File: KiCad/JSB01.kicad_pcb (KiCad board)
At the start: 2 copper layers, 88 x 33 mm, 35 parts, among them J1 MB10XX Sonar, J2 VL53LXX TOF(0x29), M1 LD14, Q2 AO3400A, SW1 Tactile, SW2 Tactile, SW3 Slide, U1 TPS61291DRVR, U2 QMC5883L(0x0D), U3 BH1750FVI(0x23)

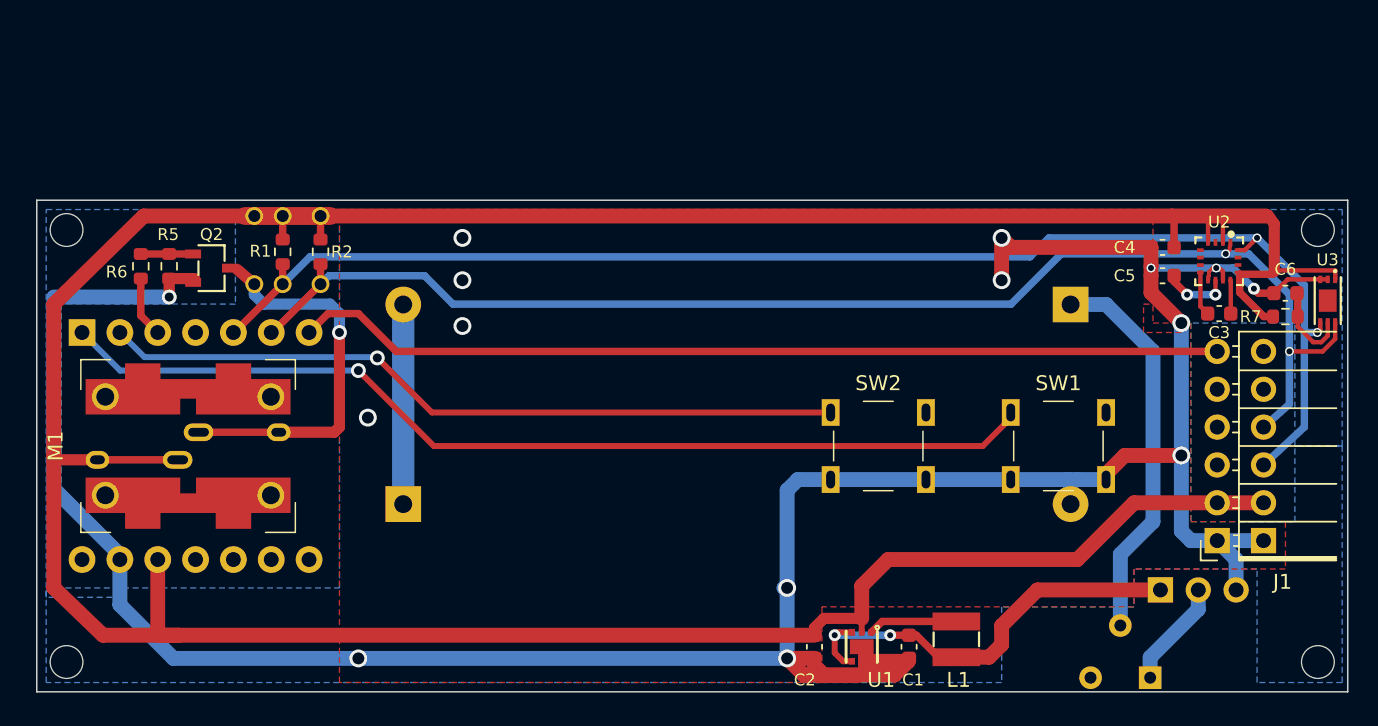
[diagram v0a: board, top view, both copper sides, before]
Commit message: BTO ver. (QMC5883P)
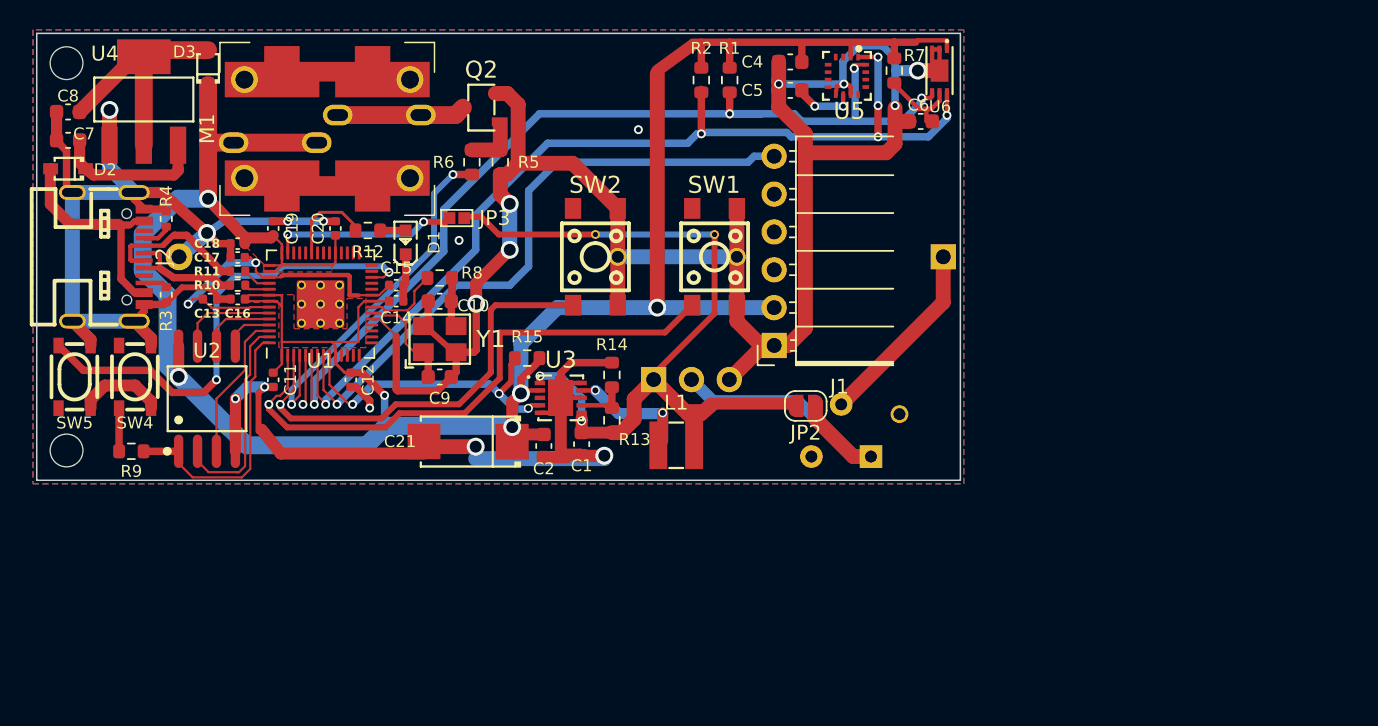
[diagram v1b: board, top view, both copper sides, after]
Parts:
- removed C3: 0.22uF, Capacitor_SMD:C_0603_1608Metric
- removed MCU1: XIAO RP2040, JSB01_Lib:MOUDLE14P-2.54-21X17.8MM
- removed the Pad at (41.9, 39.9)
- removed the Pad at (44.5, 35.4)
- removed the Pad at (40.0, 39.9)
- removed the Pad at (44.5, 39.9)
- removed the Pad at (41.9, 35.4)
- removed the Pad at (40.0, 35.4)
- removed the REF** at (27.4, 65.3)
- removed the REF** at (111.4, 65.3)
- removed the REF** at (27.4, 36.3)
- removed the REF** at (111.4, 36.3)
- added ?: , , F.Cu at (83.3, 48.8)
- added C10: 33p, Capacitor_SMD:C_0603_1608Metric, F.Cu at (52.5, 41.1)
- added C11: 100n, Capacitor_SMD:C_0402_1005Metric, F.Cu at (41.3, 46.4)
- added C12: 100n, Capacitor_SMD:C_0402_1005Metric, F.Cu at (46.5, 46.4)
- added C13: 100n, Capacitor_SMD:C_0402_1005Metric, F.Cu at (37.0, 40.9)
- added C14: 100n, Capacitor_SMD:C_0402_1005Metric, F.Cu at (49.5, 41.1)
- added C15: 100n, Capacitor_SMD:C_0402_1005Metric, F.Cu at (49.5, 40.0)
- added C16: 100n, Capacitor_SMD:C_0402_1005Metric, F.Cu at (38.9, 40.9)
- added C17: 100n, Capacitor_SMD:C_0402_1005Metric, F.Cu at (38.9, 38.1)
- added C18: 100n, Capacitor_SMD:C_0402_1005Metric, F.Cu at (38.9, 37.2)
- added C19: 100n, Capacitor_SMD:C_0402_1005Metric, F.Cu at (41.3, 36.2)
- added C20: 100n, Capacitor_SMD:C_0402_1005Metric, F.Cu at (45.5, 36.2)
- added C21: 100u, JSB01_Lib:CAP-SMD_L6.0-W3.2, F.Cu at (54.4, 50.5)
- added C7: 10u, Capacitor_SMD:C_0603_1608Metric, F.Cu at (27.5, 30.3)
- added C8: 10u, Capacitor_SMD:C_0603_1608Metric, F.Cu at (27.5, 28.4)
- added C9: 33p, Capacitor_SMD:C_0603_1608Metric, F.Cu at (52.5, 46.2)
- added D1: LED, JSB01_Lib:LED0603-RD_GREEN, F.Cu at (50.2, 37.1)
- added D2: NSR0320MW2T1G, JSB01_Lib:SOD-323_L1.8-W1.3-LS2.5-RD, F.Cu at (27.5, 32.2)
- added D3: 1N5819WS, JSB01_Lib:SOD-323_L1.8-W1.3-LS2.5-RD, F.Cu at (36.9, 25.4)
- added JP2: SolderJumper_2_Open, Jumper:SolderJumper-2_P1.3mm_Open_RoundedPad1.0x1.5mm, F.Cu at (77.0, 48.1)
- added JP3: SolderJumper_2_Open, JSB01_Lib:SolderJumper-2_Open_mini, F.Cu at (53.6, 35.5)
- added Pad: Pad1.2_0.8, JSB01_Lib:Pad1.2_0.8, F.Cu at (71.1, 38.1)
- added Pad: Pad0.6_0.35, JSB01_Lib:Pad0.6_0.35, F.Cu at (62.5, 36.6)
- added Pad: Pad0.6_0.35, JSB01_Lib:Pad0.6_0.35, F.Cu at (70.6, 36.6)
- added Pad: Pad1.2_0.8, JSB01_Lib:Pad1.2_0.8, F.Cu at (63.0, 38.1)
- added R10: 27.4, Resistor_SMD:R_0402_1005Metric, F.Cu at (38.9, 40.0)
- added R11: 27.4, Resistor_SMD:R_0402_1005Metric, F.Cu at (38.9, 39.1)
- added R12: 470, Resistor_SMD:R_0603_1608Metric, F.Cu at (47.6, 36.3)
- added R13: 470K, Resistor_SMD:R_0603_1608Metric, F.Cu at (64.0, 49.1)
- added R14: 390K, Resistor_SMD:R_0603_1608Metric, F.Cu at (64.0, 46.0)
- added R15: 1M, Resistor_SMD:R_0603_1608Metric, F.Cu at (58.3, 44.9)
- added R3: 5.1K, Resistor_SMD:R_0402_1005Metric, F.Cu at (34.1, 40.6)
- added R4: 5.1K, Resistor_SMD:R_0402_1005Metric, F.Cu at (34.1, 35.6)
- added R8: 1K, Resistor_SMD:R_0603_1608Metric, F.Cu at (52.5, 39.5)
- added R9: 1k, Resistor_SMD:R_0603_1608Metric, F.Cu at (31.8, 51.2)
- added REF**: MountingHole_2.2mm_M2, MountingHole:MountingHole_2.2mm_M2, F.Cu at (27.4, 25.1)
- added REF**: MountingHole_2.2mm_M2, MountingHole:MountingHole_2.2mm_M2, F.Cu at (27.4, 51.1)
- added SW4: SKRPABE010, JSB01_Lib:KEY-SMD_4P-L4.2-W3.2, F.Cu at (32.0, 46.2)
- added SW5: SKRPABE010, JSB01_Lib:KEY-SMD_4P-L4.2-W3.2, F.Cu at (27.9, 46.2)
- added U3: TPS61025DRCR, JSB01_Lib:VSON-10_L3.0-W3.0-P0.50-BL-EP, F.Cu at (60.6, 47.6)
- added U4: AMS1117-3.3, JSB01_Lib:SOT-223-3_L6.5-W3.4, F.Cu at (32.6, 27.6)
- added U5: QMC5883P(0x2C), JSB01_Lib:LGA-16_L3.0-W3.0-P0.50-BL_SQ, F.Cu at (79.8, 26.0)
- added Y1: TAXM12M4RLBDDT2T, JSB01_Lib:OSC-SMD_4P-L3.2-W2.5, F.Cu at (52.5, 43.6)
- BT1: value 2xAAA -> 1xAAA; footprint JSB01_Lib:BatteryHolder 2xAAA -> JSB01_Lib:BatteryHolder_SN4_1PC
- C1: value 10uF -> 10u
- C2: value 22uF -> 2.2u
- C4: value 0.1uF -> 0.1u
- C5: value 4.7uF -> 4.7u
- C6: value 1uF -> 1u
- J2: value VL53LXX TOF(0x29) -> USB_C_Receptacle_USB2.0; footprint Connector_PinSocket_2.54mm:PinSocket_1x06_P2.54mm_Vertical -> JSB01_Lib:USB-C-SMD_TYPE-C-16P-1; moved to F.Cu
- L1: value 3.3μH -> 6.8μH
- R1, R2: value 10KΩ -> 4.7K
- R5: value 100KΩ -> 100K
- R6: value 20KΩ -> 20K
- SW1, SW2: footprint JSB01_Lib:SW_tactile_DTS6 -> JSB01_Lib:SW-SMD_4P-L4.5-W4.5-P3.00-LS6.8
- U1: value TPS61291DRVR -> RP2040; footprint JSB01_Lib:WSON-6_L2.0-W2.0-P0.65-BL-EP -> JSB01_Lib:RP2040-QFN-56
- U2: value QMC5883L(0x0D) -> W25Q128JVSIQ; footprint JSB01_Lib:LGA-16_L3.0-W3.0-P0.50-BL_SQ -> JSB01_Lib:SOP-8-208mil
- moved J2 79.9 mm to (30.2, 38.1), turned to -90 degrees
- moved U2 68.6 mm to (36.8, 47.6), turned to 0 degrees
- moved U1 43.0 mm to (44.5, 41.3), turned to 90 degrees
- moved JP1 36.8 mm to (69.3, 46.3)
- moved J1 32.5 mm to (74.9, 37.7)
- moved R1 32.1 mm to (71.9, 26.2)
- moved R7 31.0 mm to (83.0, 25.6), turned to -90 degrees
- moved U6 30.3 mm to (86.0, 25.6)
- moved R2 28.0 mm to (70.0, 26.2)
- moved C4 27.9 mm to (76.0, 25.0)
- moved C5 27.9 mm to (76.0, 26.9)
- moved C6 27.1 mm to (84.7, 29.0)
- moved SW1 26.3 mm to (70.9, 38.1), turned to 90 degrees
- moved C1 25.8 mm to (62.0, 50.7)
- moved SW3 23.9 mm to (79.4, 49.8)
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- renumbered U3 to U6
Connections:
- C2 pad 1: +3.3V -> +3V3
- C4 pad 1: +3.3V -> +3V3
- C5 pad 1: Net-(U2-C1) -> Net-(U5-C1)
- J1 pad 2: +3.3V -> +3V3
- J1 pad 6: Net-(J1-PW) -> SONAR_PW
- L1 pad 2: Net-(U1-SW) -> Net-(U3-SW)
- M1 pad 1: +3.3V -> +3V3
- R1 pad 1: +3.3V -> +3V3
- R1 pad 2: Net-(J2-SDA) -> SDA
- R2 pad 1: +3.3V -> +3V3
- R2 pad 2: Net-(J2-SCL) -> SCL
- R6 pad 1: Net-(MCU1-D2) -> VIB
- R7 pad 1: +3.3V -> +3V3
- SW1 pad 1: Net-(MCU1-D0) -> SW1
- SW1 pad 2: GND -> SW1
- SW2 pad 1: Net-(MCU1-D1) -> SW2
- SW2 pad 2: GND -> SW2
- U1 pad 1: Net-(U1-SW) -> +3V3
- U1 pad 2: +3.3V -> SW1
- U1 pad 3: Net-(JP1-A) -> SW2
- U1 pad 4: Net-(JP1-A) -> VIB
- U1 pad 5: GND -> unconnected-(U1-GPIO3-Pad5)
- U1 pad 6: GND -> SDA
- U1 pad 7: GND -> SCL
- U2 pad 1: Net-(J2-SCL) -> QSPI_SS
- U2 pad 2: +3.3V -> QSPI_SD1
- U2 pad 3: unconnected-(U2-Pad3) -> QSPI_SD2
- U2 pad 4: +3.3V -> GND
- U2 pad 5: unconnected-(U2-Pad5) -> QSPI_SD0
- U2 pad 6: unconnected-(U2-Pad6) -> QSPI_SCLK
- U2 pad 7: unconnected-(U2-Pad7) -> QSPI_SD3
- U2 pad 8: Net-(U2-SETP) -> +3V3
- U6 pad 1: +3.3V -> +3V3
- U6 pad 4: Net-(J2-SDA) -> SDA
- U6 pad 6: Net-(J2-SCL) -> SCL
- U6 pad 7: unconnected-(U3-EP-Pad7) -> GND
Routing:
- net +3.3V: track 228.7 -> 0.00 mm
- net +3V3: track 0.00 -> 177.1 mm, vias 0 -> 6
- net Net-(J2-SDA): track 93.8 -> 0.00 mm, vias 2 -> 0
- net Net-(J2-SCL): track 89.9 -> 0.00 mm, vias 2 -> 0
- net Net-(MCU1-D0): track 66.7 -> 0.00 mm, vias 1 -> 0
- net SCL: track 0.00 -> 66.3 mm, vias 0 -> 6
- net SDA: track 0.00 -> 64.5 mm, vias 0 -> 4
- net Net-(J1-PW): track 62.5 -> 0.00 mm
- net GND: track 198.1 -> 253.9 mm, vias 15 -> 18
- net Net-(MCU1-D1): track 49.9 -> 0.00 mm, vias 1 -> 0
- net SONAR_PW: track 0.00 -> 43.2 mm, vias 0 -> 1
- net SW1: track 0.00 -> 38.4 mm, vias 0 -> 1
- net RESET: track 0.00 -> 31.8 mm, vias 0 -> 2
- net SW2: track 0.00 -> 29.5 mm, vias 0 -> 1
- net Net-(JP1-A): track 29.0 -> 56.6 mm
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- added copper zone on F.Cu, net +3V3
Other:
- board size 88 x 33 mm -> 62 x 30 mm
- board text added: "JSB01 Rev 1.0"
- board text removed: "JSB01 Rev 0.1"
